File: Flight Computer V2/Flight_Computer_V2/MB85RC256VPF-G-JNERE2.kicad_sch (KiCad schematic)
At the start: 7 parts, among them IC1 MB85RC256VPF-G-JNERE2

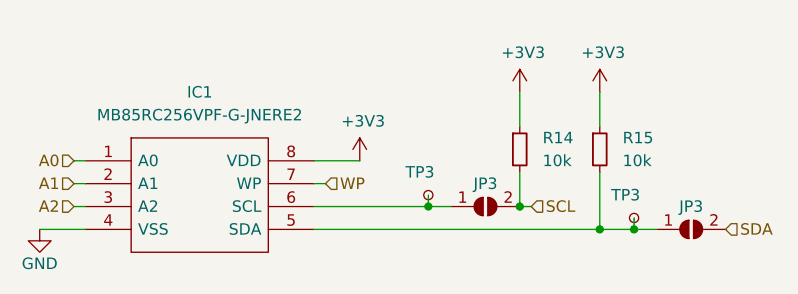
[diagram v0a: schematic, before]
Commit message: updated pcb
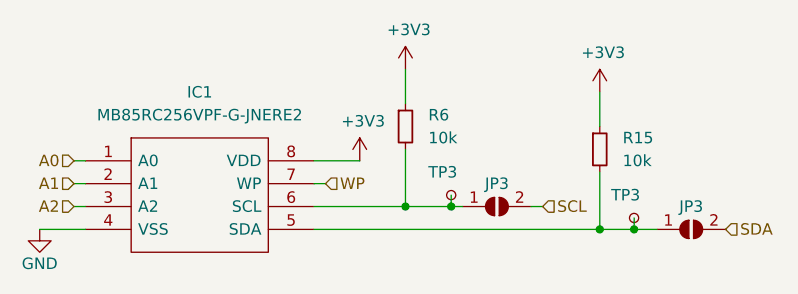
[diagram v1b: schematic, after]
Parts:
- removed R14: 10k, symbol Device:R_Small
- added R6: 10k, Resistor_SMD:R_0402_1005Metric, symbol Device:R_Small
- IC1: footprint SOIC127P798X210-8N -> LibraryLoader:SOIC127P798X210-8N
- JP3: footprint (none) -> Jumper:SolderJumper-2_P1.3mm_Open_Pad1.0x1.5mm
- R15: footprint (none) -> Resistor_SMD:R_0402_1005Metric
- TP3: footprint (none) -> TestPoint:TestPoint_Pad_D1.0mm
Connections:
- net +3V3: now also R6.1
- net at IC1.6 (SCL), JP3.1 (A), TP3.1: now also R6.2
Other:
- moved on the sheet: JP3, TP3
